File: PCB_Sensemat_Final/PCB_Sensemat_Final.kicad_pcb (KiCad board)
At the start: 4 copper layers, 70 x 65 mm, 53 parts, among them J1 teensy_ingangen_1tm24_Socket, J2 Philips_pins_1tm24, J3 Philips_pins_30tm53, J4 teensy_ingangen_25tm48_Socket, U4 DAC0_MCP4725, U5 DAC1_MCP4725, U7 ADS131M08xPBS, Y1 ASE-xxxMHz

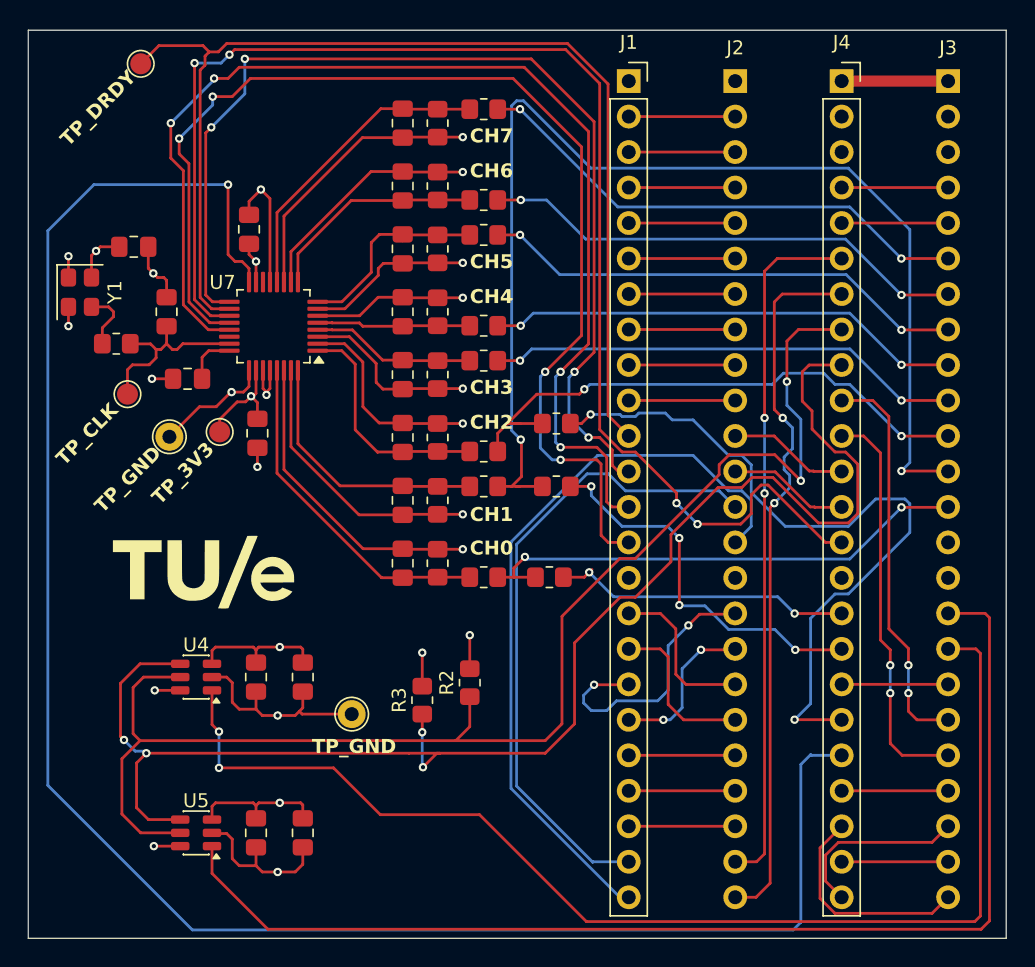
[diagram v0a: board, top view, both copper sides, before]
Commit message: PCB_Sensemat
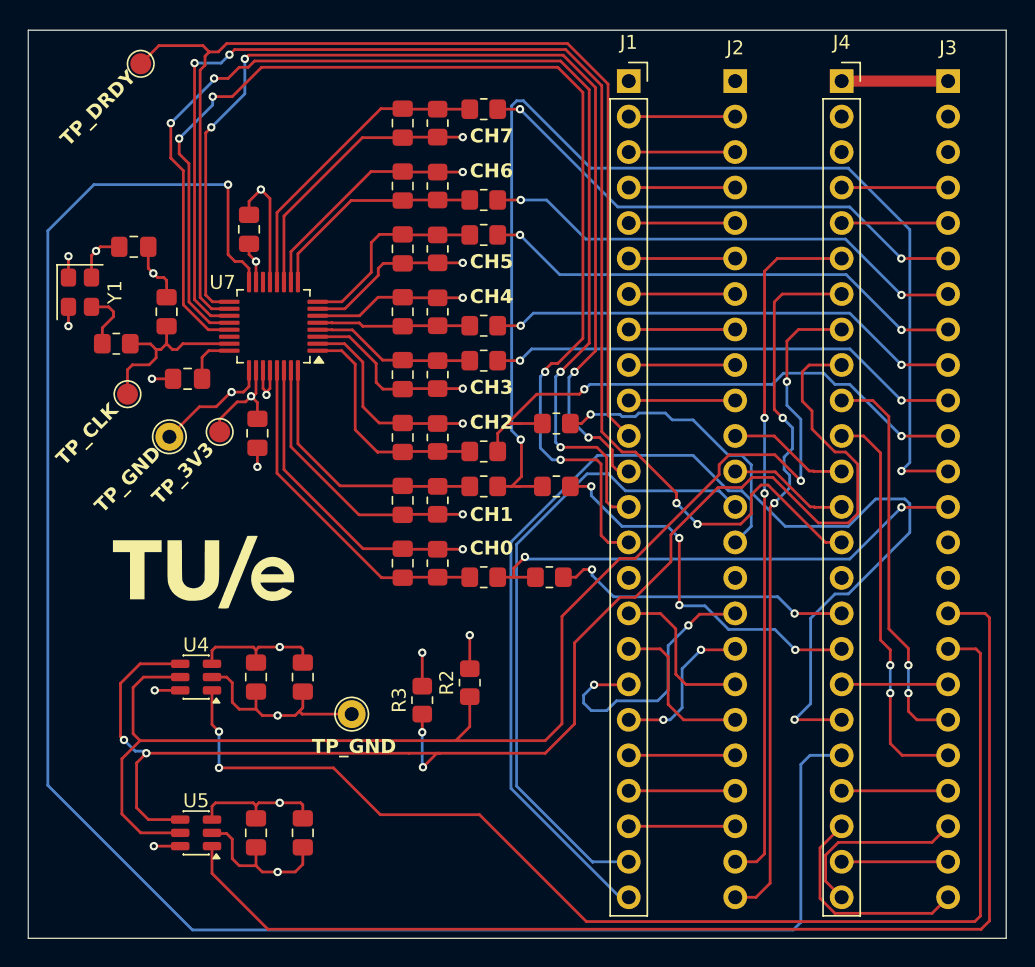
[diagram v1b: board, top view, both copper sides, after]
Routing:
- net /ADC_MISO: track 83.3 -> 86.7 mm
- net /ADC_MOSI: track 83.2 -> 85.4 mm
- net /ADC_CS: track 75.3 -> 77.1 mm
